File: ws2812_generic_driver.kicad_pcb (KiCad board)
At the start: 2 copper layers, 21 parts, among them J1 Conn_01x01, J2 Conn_01x01, J3 Conn_01x01, J4 Conn_01x01, J5 Conn_01x01, J6 Conn_01x01, J7 Conn_01x01, J8 Conn_ARM_JTAG_SWD_10, U1 ATSAMD21E15L-A, U2 TC2014-3.3VxCTTR, U3 MCP1640CH

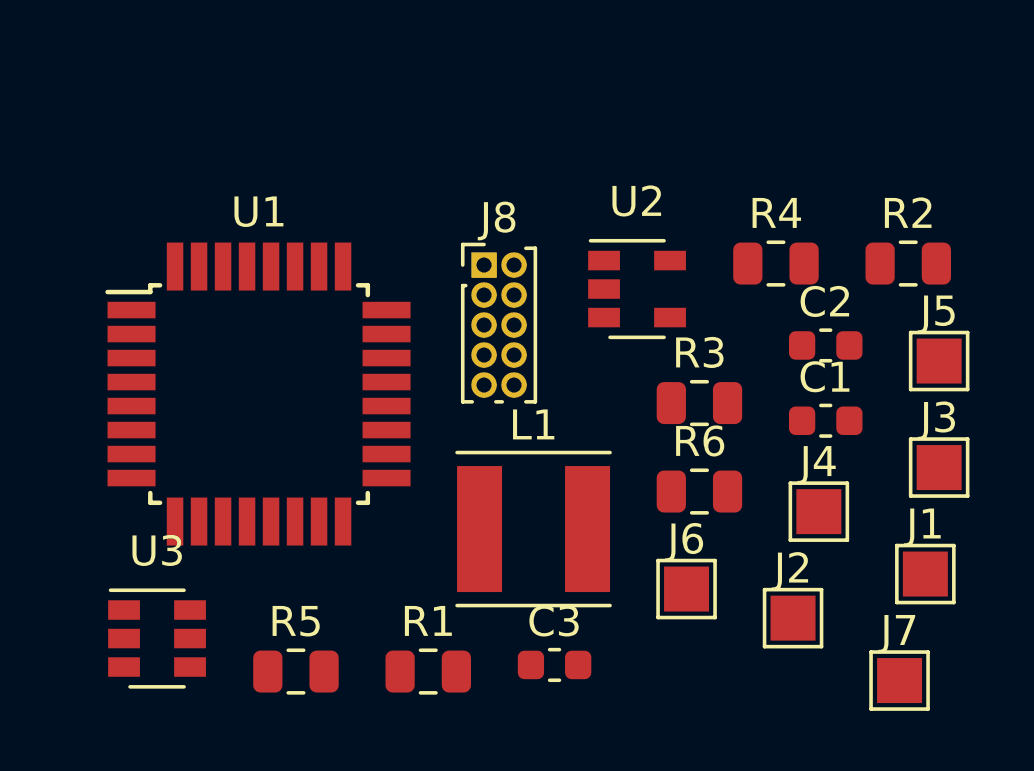
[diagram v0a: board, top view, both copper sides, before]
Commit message: Finish PCB
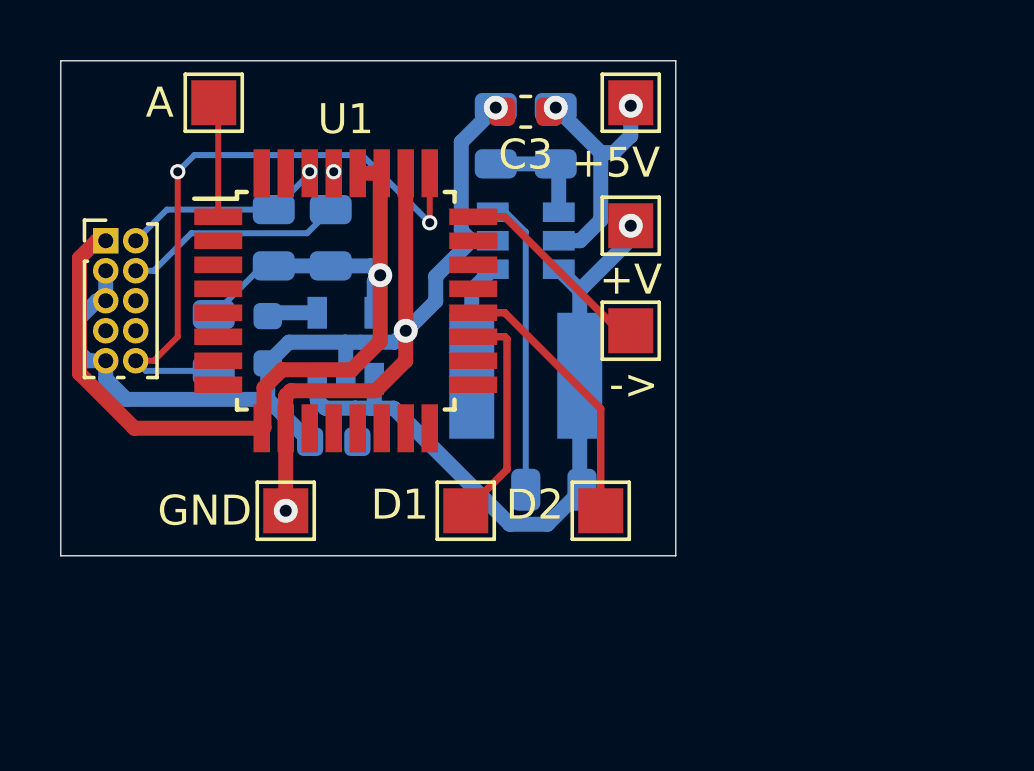
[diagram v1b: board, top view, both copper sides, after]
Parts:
- C1, C2, L1, R1, R2, R3, R4, R5, R6, U2, U3: moved to B.Cu
- moved J7 29.9 mm to (135.1, 88.4)
- moved R5 19.8 mm to (146.5, 89.5), turned to 270 degrees
- moved R2 19.3 mm to (139.0, 92.9), turned to 90 degrees
- moved C1 18.8 mm to (136.9, 96.3), turned to 270 degrees
- moved C3 18.5 mm to (145.5, 88.7), turned to 180 degrees
- moved U3 18.1 mm to (145.5, 93.0)
- moved J2 18.0 mm to (149.0, 88.4)
- moved J4 17.8 mm to (137.5, 102.0)
- moved C2 16.7 mm to (139.1, 99.7), turned to 180 degrees
- moved R3 15.2 mm to (137.1, 92.9), turned to 90 degrees
- moved J1 15.2 mm to (149.0, 92.5)
- moved R6 13.7 mm to (144.5, 89.5), turned to 90 degrees
- moved R1 13.1 mm to (135.1, 96.4), turned to 270 degrees
- moved J8 12.6 mm to (131.5, 93.0)
- moved J5 12.3 mm to (148.0, 102.0)
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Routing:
- net GND: track 0.00 -> 44.3 mm, vias 0 -> 3
- net +3.3V: track 0.00 -> 31.8 mm, vias 0 -> 1
- net +V: track 0.00 -> 24.4 mm, vias 0 -> 1
- net RESET: track 0.00 -> 21.2 mm, vias 0 -> 2
- net Net-(R4-Pad2): track 0.00 -> 9.97 mm
- net D1: track 0.00 -> 8.98 mm
- net SWCLK: track 0.00 -> 8.65 mm, vias 0 -> 1
- net +5V: track 0.00 -> 8.29 mm, vias 0 -> 2
- net D2: track 0.00 -> 7.45 mm
- net DOUT: track 0.00 -> 6.82 mm
- net SWDIO: track 0.00 -> 6.79 mm, vias 0 -> 1
- net A1: track 0.00 -> 3.86 mm
- net Net-(L1-Pad2): track 0.00 -> 3.84 mm
- net Net-(R5-Pad2): track 0.00 -> 3.65 mm
- net Net-(C1-Pad1): track 0.00 -> 1.70 mm
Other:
- board outline added: 20.5 x 16.5 mm
- board text added: "+5V"
- board text added: "+V"
- board text added: "->"
- board text added: "A"
- board text added: "D1"
- board text added: "D2"
- board text added: "GND"
